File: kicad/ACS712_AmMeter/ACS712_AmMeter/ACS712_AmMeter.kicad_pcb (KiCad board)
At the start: 2 copper layers, 94 x 71.1 mm, 37 parts, among them J1 BATT_IN, J2 GND, J3 I2C_PIN, J4 POS_IN, J5 NEG_IN, U1 NJM2396, U2 TLE2426xLP, U3 OLED_SSD1306_I2C, U4 NJU7032D

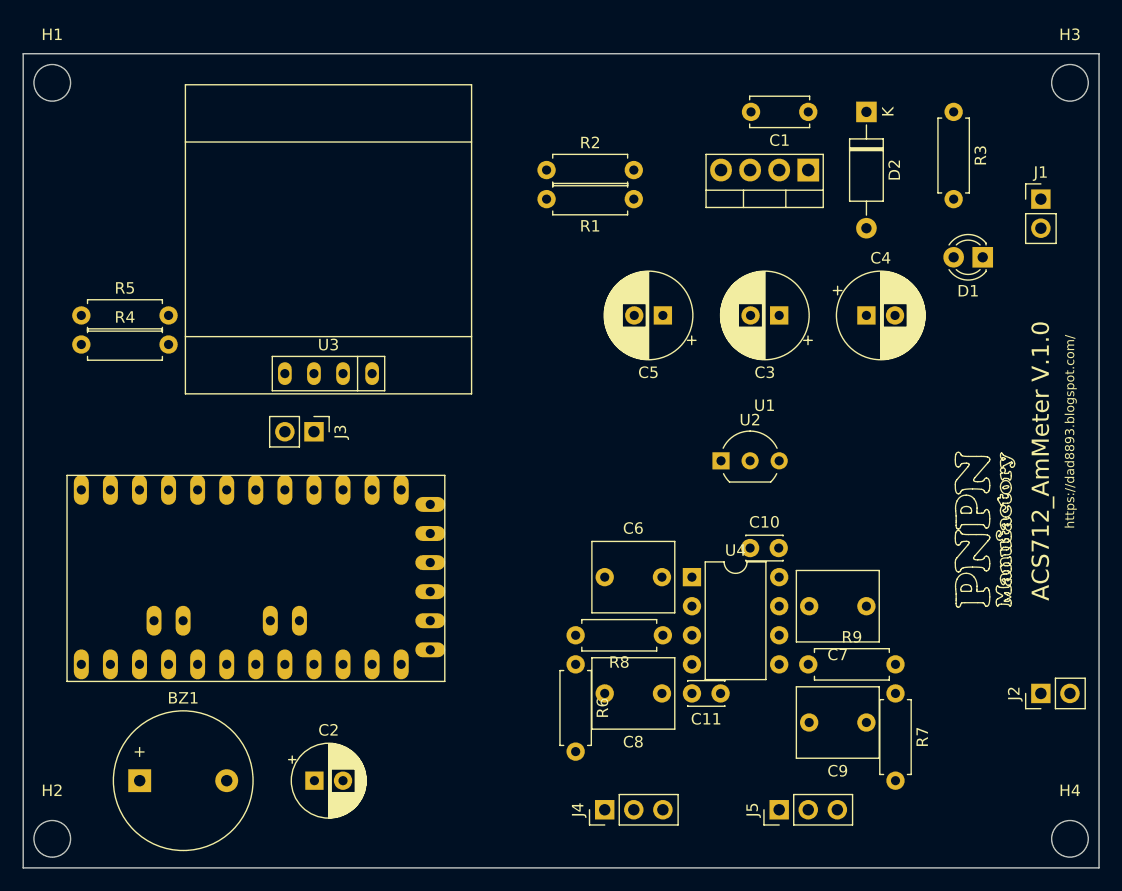
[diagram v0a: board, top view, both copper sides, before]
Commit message: Add: logo bule, Update: KiCad design
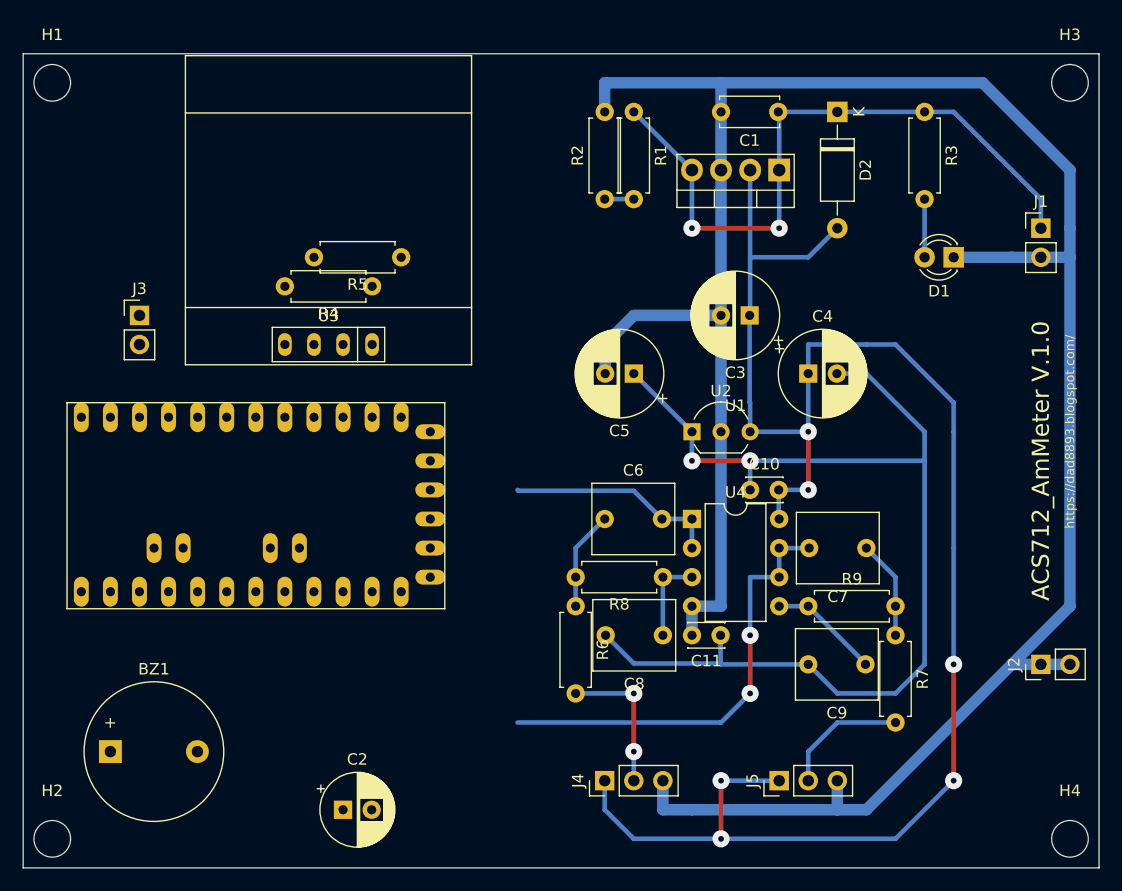
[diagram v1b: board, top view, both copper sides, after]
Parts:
- moved R5 28.4 mm to (132.1, 78.7), turned to 180 degrees
- moved R4 25.9 mm to (129.5, 81.3), turned to 180 degrees
- moved J3 18.3 mm to (109.2, 83.8), turned to 0 degrees
- moved R1 7.62 mm to (152.4, 66.0), turned to 270 degrees
- moved C4 7.18 mm to (167.6, 88.9)
- moved A1 6.35 mm to (119.4, 101.6)
- moved C5 5.68 mm to (152.4, 88.9)
- moved R2 5.68 mm to (149.9, 73.7), turned to 90 degrees
- moved C8 5.08 mm to (154.9, 111.8)
- moved C9 5.08 mm to (172.6, 114.3)
- moved C6 5.08 mm to (149.9, 101.6)
- moved U4 5.08 mm to (157.5, 101.6)
- moved C10 5.08 mm to (162.6, 99.1)
- moved C11 5.08 mm to (160.0, 111.8)
- moved C7 5.08 mm to (172.7, 104.1)
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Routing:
- net GND: track 0.00 -> 212.2 mm
- net +5V: track 0.00 -> 148.6 mm, vias 0 -> 6
- net +2V5: track 0.00 -> 96.2 mm, vias 0 -> 2
- net +BATT: track 0.00 -> 58.7 mm, vias 0 -> 2
- net V_NEG: track 0.00 -> 39.2 mm, vias 0 -> 2
- net V_POS: track 0.00 -> 18.8 mm
- net Net-(J4-Pad2): track 0.00 -> 12.7 mm, vias 0 -> 2
- net Net-(J5-Pad2): track 0.00 -> 11.2 mm
- net Net-(C9-Pad1): track 0.00 -> 9.80 mm
- net Net-(C6-Pad1): track 0.00 -> 8.67 mm
- net Net-(C7-Pad1): track 0.00 -> 8.67 mm
- net Net-(C8-Pad1): track 0.00 -> 7.62 mm
- net Net-(D1-Pad2): track 0.00 -> 5.08 mm
- net V_BATT: track 0.00 -> 2.54 mm
